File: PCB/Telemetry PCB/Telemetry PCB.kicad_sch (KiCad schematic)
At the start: 35 parts, among them IC1 E22-900M22S, J1 Conn_01x04_Pin, J2 GPS, J3 Batt, SW1 SW_MEC_5E, SW2 SW_MEC_5E, U1 STM32F411CEUx, U2 AP62200WU, Y1 25MHZ 9pF, Y2 32.768k 6pF

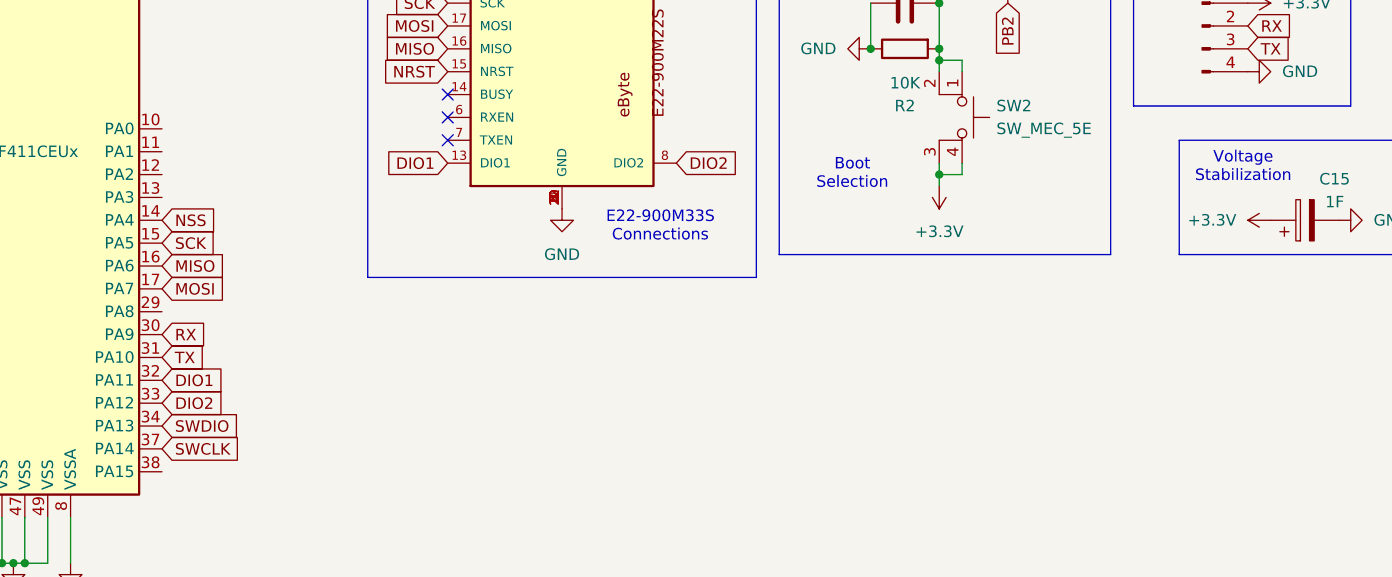
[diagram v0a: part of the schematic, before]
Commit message: more footprints
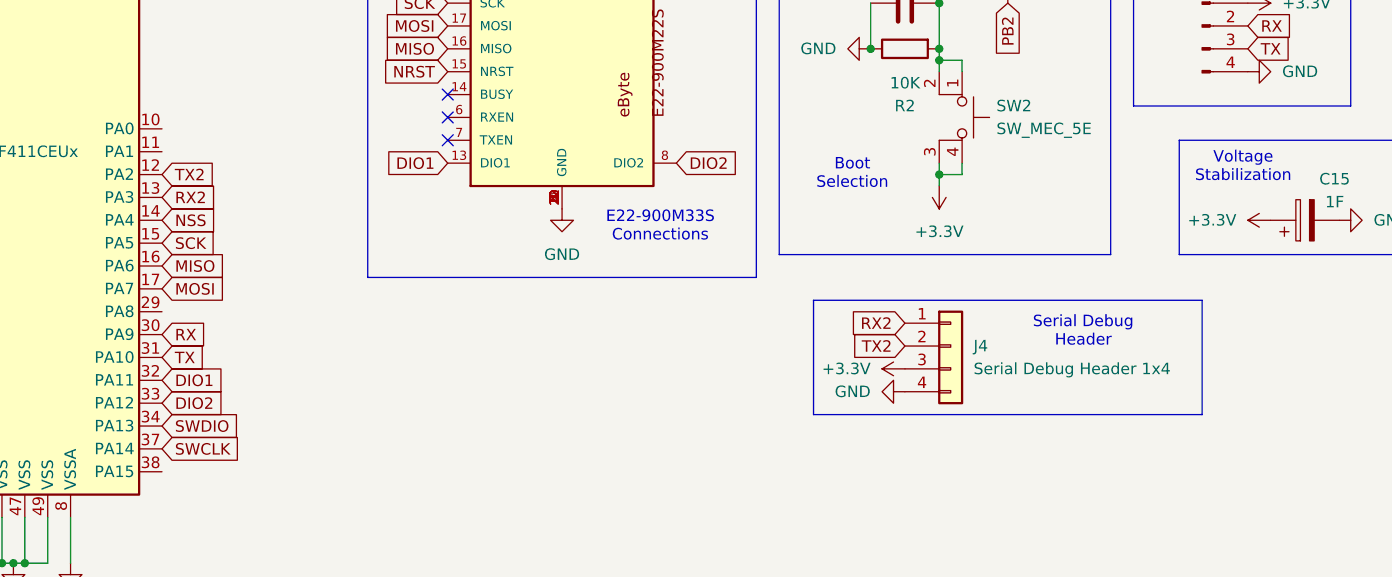
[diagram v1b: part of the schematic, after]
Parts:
- added J4: Serial Debug Header 1x4, Connector_PinHeader_2.54mm:PinHeader_1x04_P2.54mm_Vertical, symbol Connector_Generic:Conn_01x04
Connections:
- net +3.3V: now also J4.3 (Pin_3)
- net GND: now also J4.4 (Pin_4)
- net TX2: now reaches U1.12 (PA2)
- net TX2: now also J4.2 (Pin_2)
- net RX2: now reaches U1.13 (PA3)
- net RX2: now also J4.1 (Pin_1)
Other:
- note added: "Serial Debug Header"
